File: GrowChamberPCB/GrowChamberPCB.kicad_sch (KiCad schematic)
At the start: 82 parts, among them J1 Screw_Terminal_01x02, J11 Conn_01x24_Pin, J3 TYPE-C-31-M-12, J7 Screw_Terminal_01x05, J8 Screw_Terminal_01x02, Q1 IRLML6244, Q2 IRLML6244, Q3 IRLML6244, Q4 IRLML6244, Q5 IRLML6244, Q6 IRLML6244, Q7 IRLR8721, Q8 IRLML6244, SW2 Reset, SW5 BootSwitch, U1 ESP32-S3-WROOM-1U, U2 MCP1826S, U3 USBLC6-2SC6, U4 TC4428xOA, U5 W25Q128JVS, U6 CR2013-MI2120

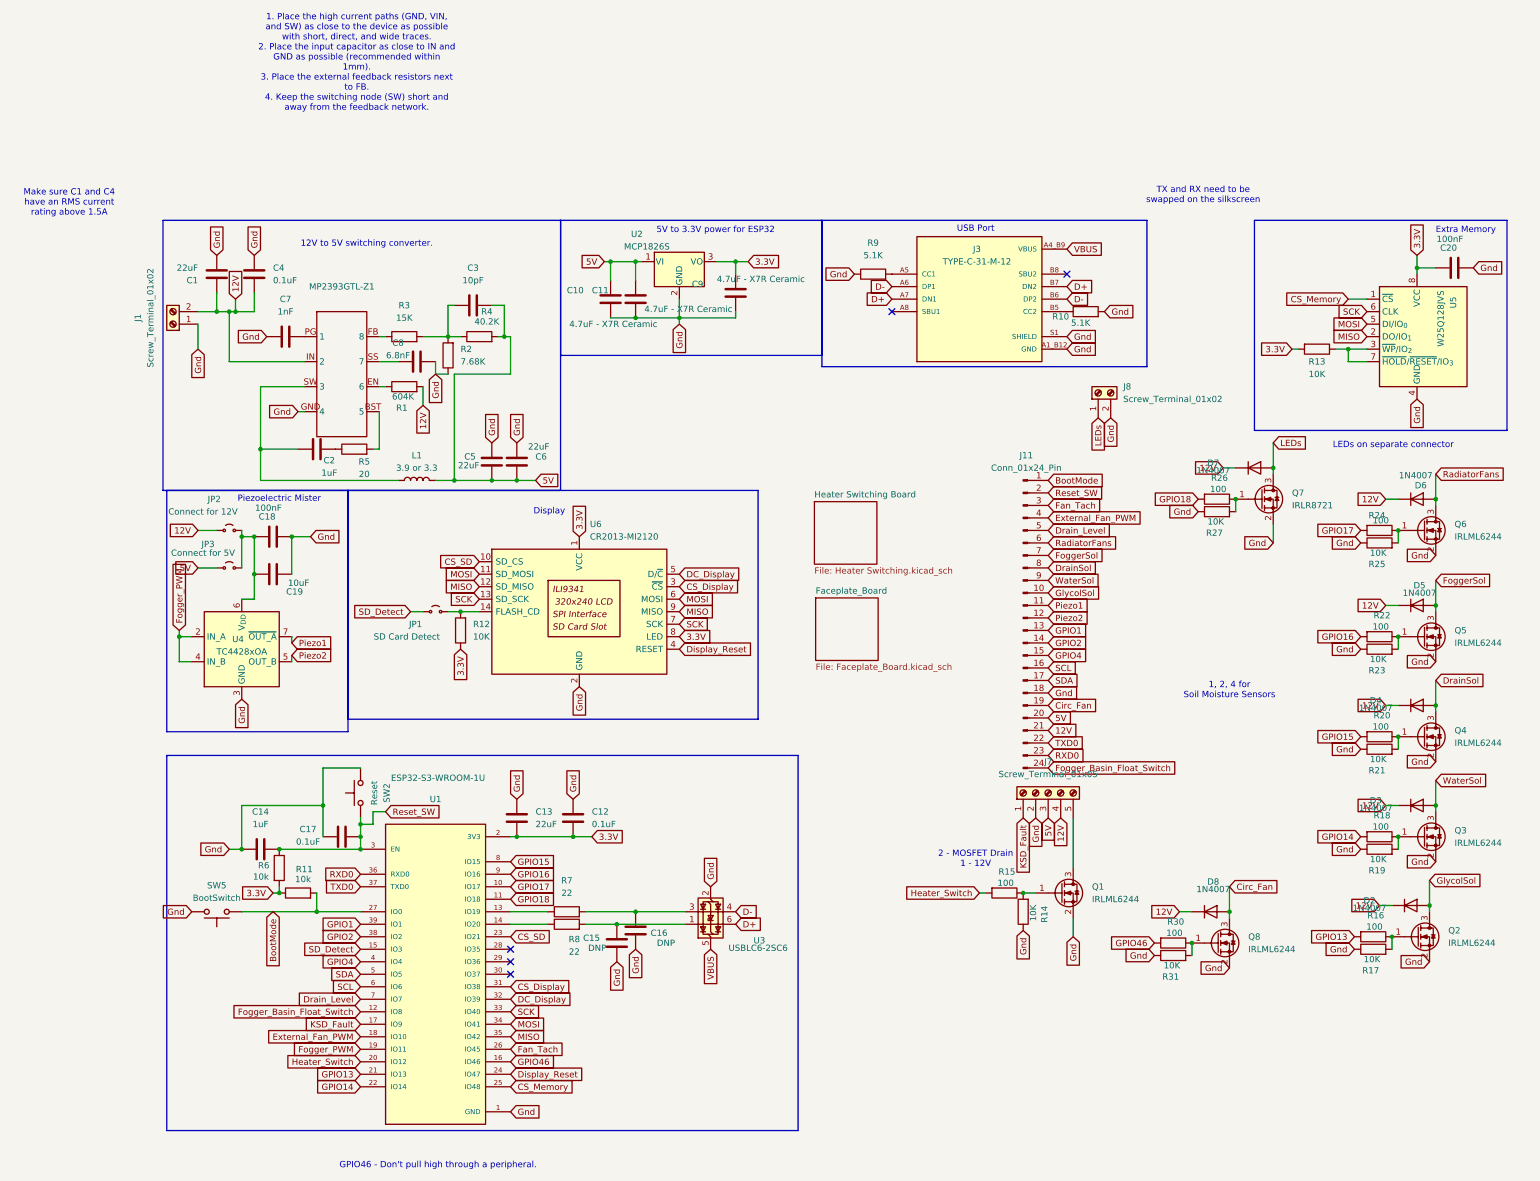
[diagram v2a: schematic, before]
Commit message: Assigning footprints and stuff
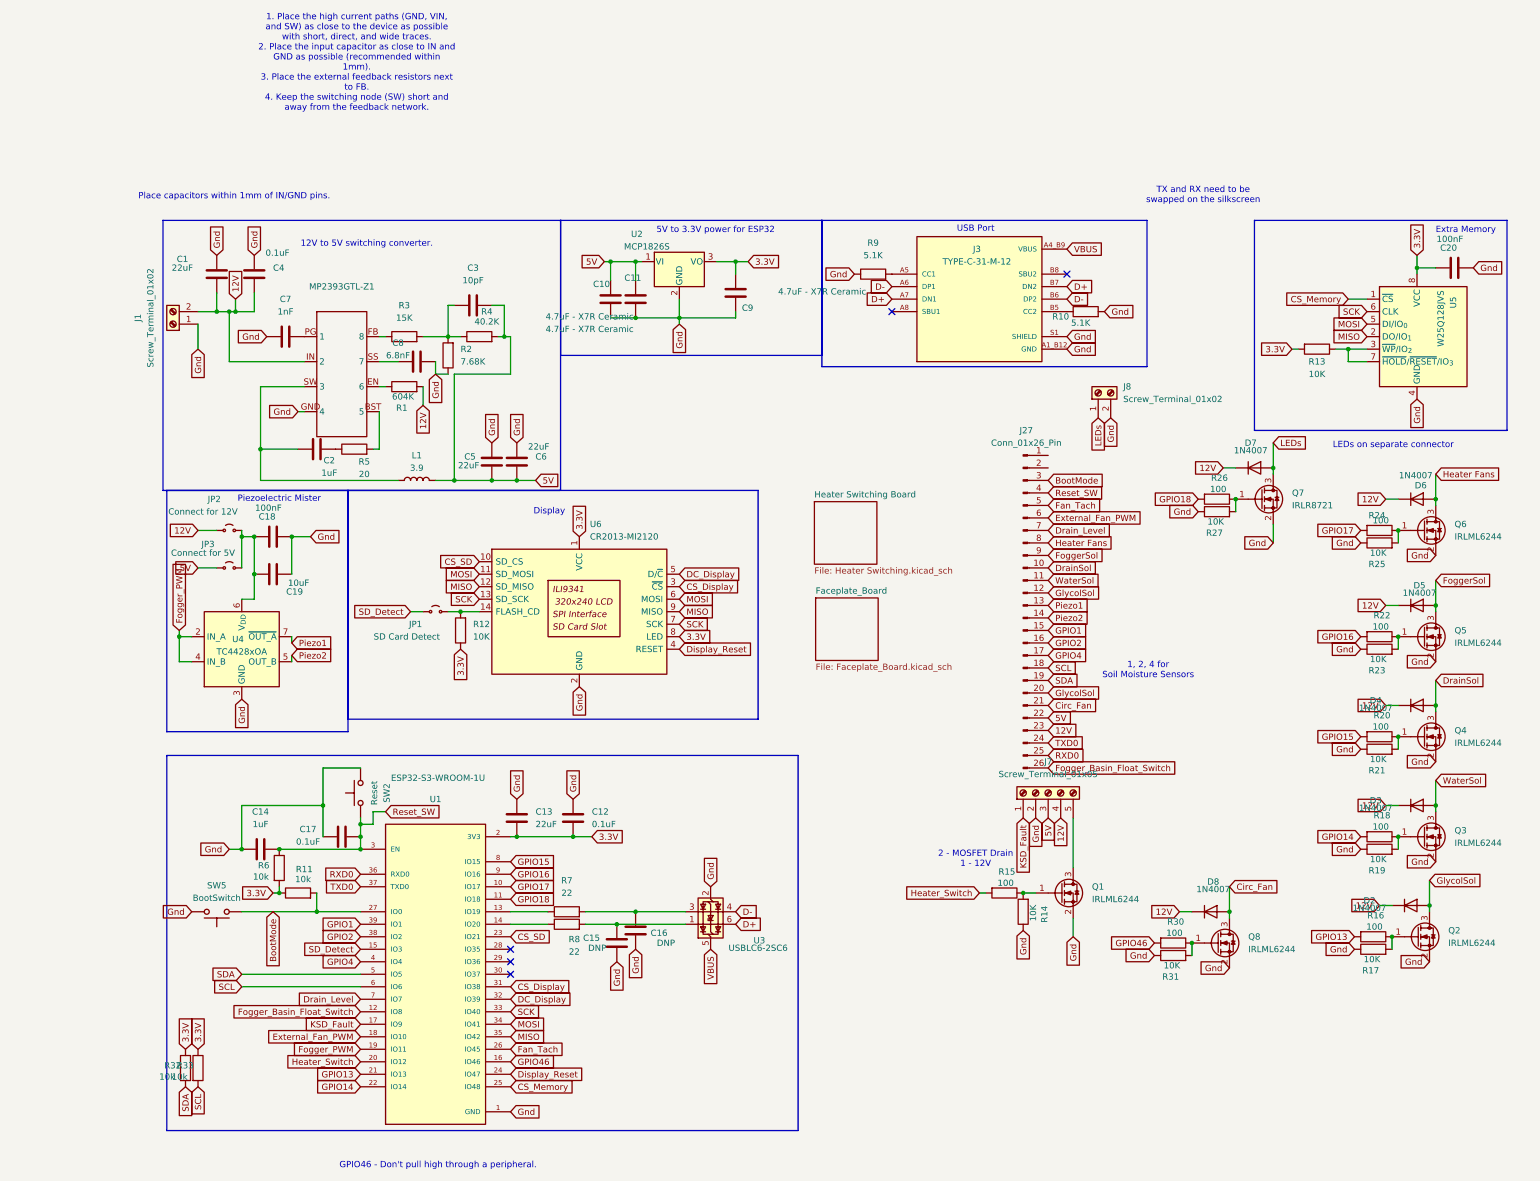
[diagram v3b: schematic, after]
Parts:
- removed J11: Conn_01x24_Pin, symbol Connector:Conn_01x24_Pin
- added J27: Conn_01x26_Pin, symbol Connector:Conn_01x26_Pin
- added R32, R33: 10k, symbol Device:R
- C1: footprint (none) -> Capacitor_SMD:C_0805_2012Metric; MFG Part Number (none) -> GRM21BR61E226ME44L; Type (SMD/thru-hole, etc.) (none) -> SMD
- C4: footprint (none) -> Capacitor_SMD:C_0603_1608Metric; MFG Part Number (none) -> GRM188R71C105KA12D
- J3: Package Package -> (none); Package/Footprint (none) -> Package
- L1: value 3.9 or 3.3 -> 3.9
- U1: Package SMD-41 Espressif Systems -> (none); Package/Footprint (none) -> SMD-41 Espressif Systems
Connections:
- net 12V: now also J27.23 (Pin_23)
- net 3.3V: now also R32.1, R33.1
- net 5V: now also J27.22 (Pin_22)
- net BootMode: now also J27.3 (Pin_3)
- net Circ_Fan: now also J27.21 (Pin_21)
- net DrainSol: now also J27.10 (Pin_10)
- net Drain_Level: now also J27.7 (Pin_7)
- net External_Fan_PWM: now also J27.6 (Pin_6)
- net Fan_Tach: now also J27.5 (Pin_5)
- net FoggerSol: now also J27.9 (Pin_9)
- net Fogger_Basin_Float_Switch: now also J27.26 (Pin_26)
- net GPIO1: now also J27.15 (Pin_15)
- net GPIO2: now also J27.16 (Pin_16)
- net GPIO4: now also J27.17 (Pin_17)
- net GlycolSol: now also J27.12 (Pin_12), J27.20 (Pin_20)
- net Piezo1: now also J27.13 (Pin_13)
- net Piezo2: now also J27.14 (Pin_14)
- net RXD0: now also J27.25 (Pin_25)
- net Reset_SW: now also J27.4 (Pin_4)
- net SCL: now also J27.18 (Pin_18), R33.2
- net SDA: now also J27.19 (Pin_19), R32.2
- net TXD0: now also J27.24 (Pin_24)
- net WaterSol: now also J27.11 (Pin_11)
- net RadiatorFans renamed Heater Fans
- net Heater Fans: now also J27.8 (Pin_8)
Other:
- note added: "Place capacitors within 1mm of IN/GND pins."
- note removed: "Make sure C1 and C4 have an RMS current rating above 1.5A"
